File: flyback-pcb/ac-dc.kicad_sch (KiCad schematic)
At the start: 12 parts, among them U2 CAP200DG

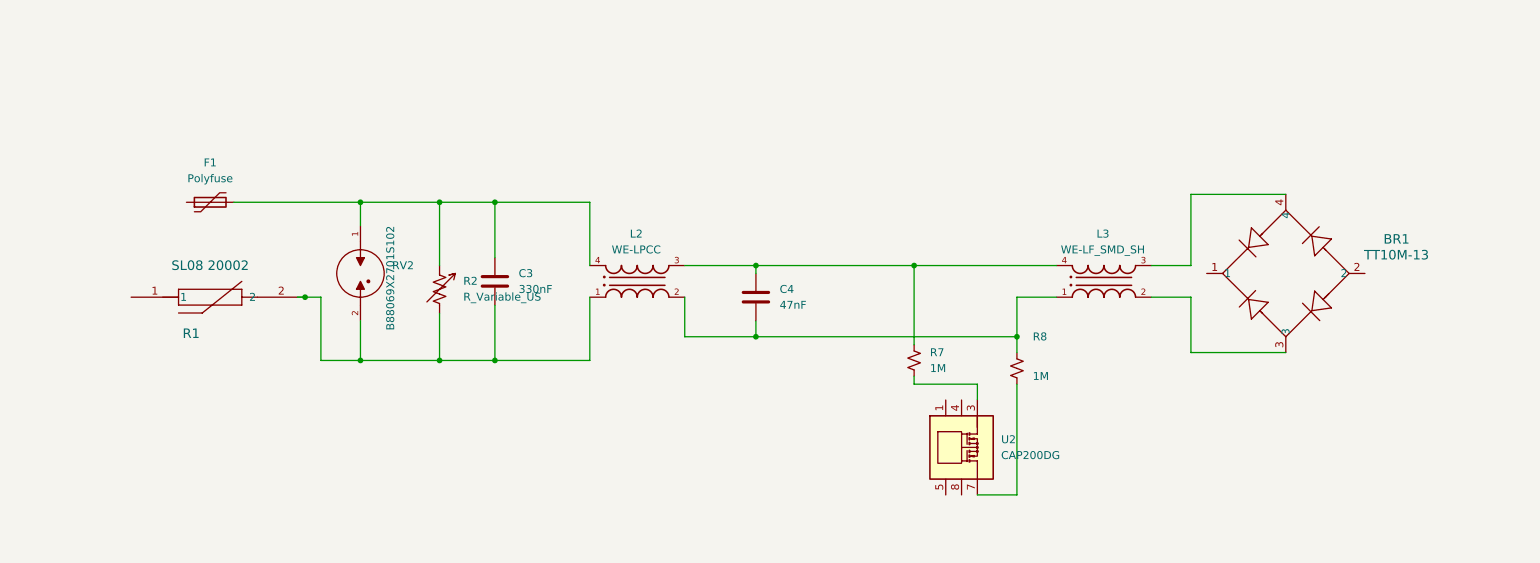
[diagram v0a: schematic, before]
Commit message: Re-done ac-dc
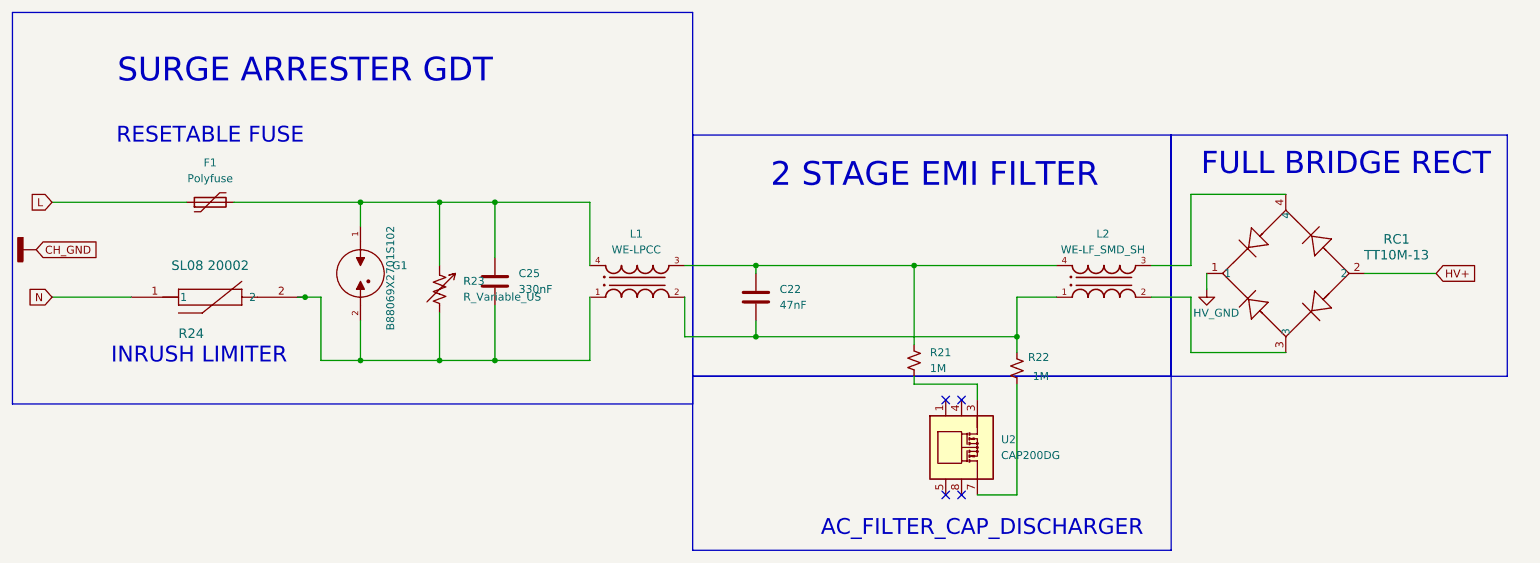
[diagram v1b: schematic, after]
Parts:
- renumbered C4 to C22, C3 to C25, RV2 to G1, L2 to L1, L3 to L2, R7 to R21, R8 to R22, R2 to R23, R1 to R24, BR1 to RC1
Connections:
- net N: now reaches R24.1
- net HV_GND: now reaches RC1.1
- net HV+: now reaches RC1.2
- net L: now reaches F1.1
- no-connect marks 0 -> 4
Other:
- note added: "2 STAGE EMI FILTER"
- note added: "AC_FILTER_CAP_DISCHARGER"
- note added: "FULL BRIDGE RECT"
- note added: "INRUSH LIMITER"
- note added: "RESETABLE FUSE"
- note added: "SURGE ARRESTER GDT"
